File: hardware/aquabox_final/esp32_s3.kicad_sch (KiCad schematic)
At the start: 16 parts, among them J3 TFT - 1.8{dblquote} SPI, SW1 BOMBA, SW2 MANUAL?AUTOMATICO, U2 ESP32-S3-DEVKITC-1-N16R8V

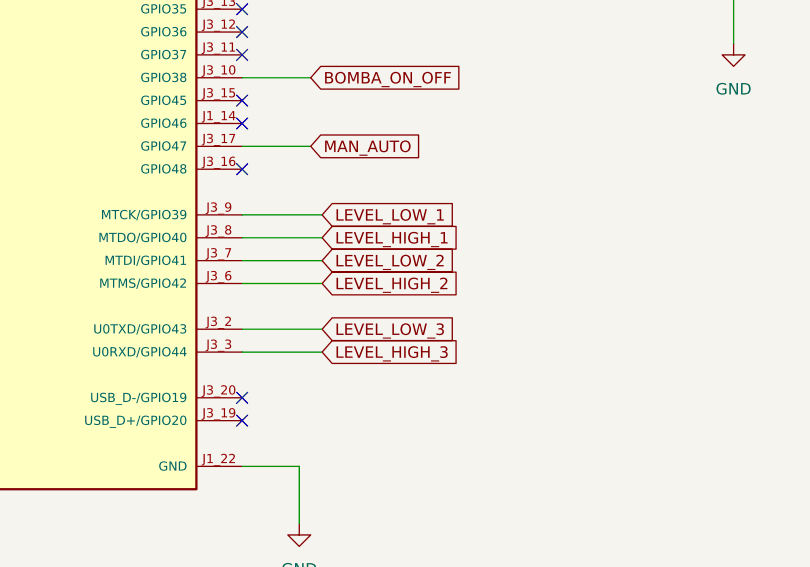
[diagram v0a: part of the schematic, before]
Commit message: Atualização
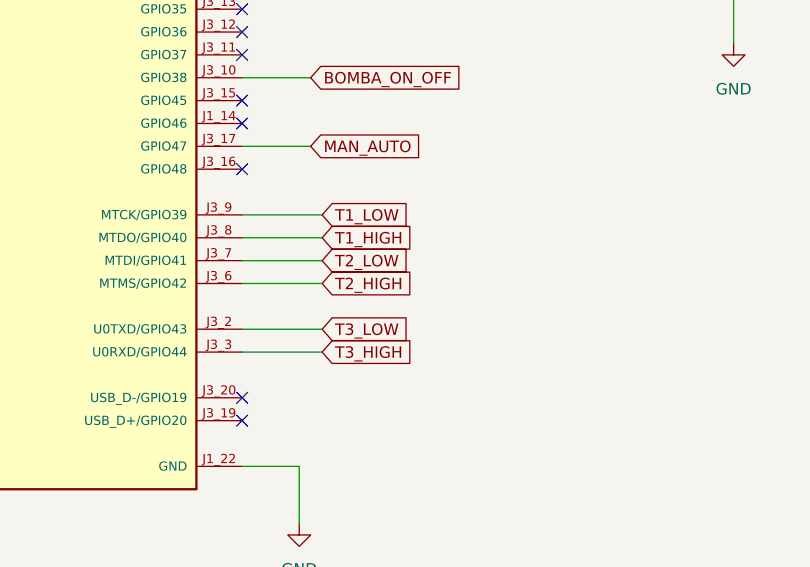
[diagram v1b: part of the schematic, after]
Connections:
- net LEVEL_HIGH_1 renamed T1_HIGH
- net LEVEL_HIGH_2 renamed T2_HIGH
- net LEVEL_HIGH_3 renamed T3_HIGH
- net LEVEL_LOW_1 renamed T1_LOW
- net LEVEL_LOW_2 renamed T2_LOW
- net LEVEL_LOW_3 renamed T3_LOW
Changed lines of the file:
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@@
 		)
 	)
-	(global_label "LEVEL_HIGH_3"
+	(global_label "T3_HIGH"
 		(shape input)
 		(at 176.53 116.84 0)
@@
 		)
 	)
-	(global_label "LEVEL_LOW_2"
+	(global_label "T2_LOW"
 		(shape input)
 		(at 176.53 106.68 0)
@@
 		)
 	)
-	(global_label "LEVEL_HIGH_1"
+	(global_label "T1_HIGH"
 		(shape input)
 		(at 176.53 104.14 0)
@@
 		)
 	)
-	(global_label "LEVEL_LOW_1"
+	(global_label "T1_LOW"
 		(shape input)
 		(at 176.53 101.6 0)
@@
 		)
 	)
-	(global_label "LEVEL_HIGH_2"
+	(global_label "T2_HIGH"
 		(shape input)
 		(at 176.53 109.22 0)
@@
 		)
 	)
-	(global_label "LEVEL_LOW_3"
+	(global_label "T3_LOW"
 		(shape input)
 		(at 176.53 114.3 0)
